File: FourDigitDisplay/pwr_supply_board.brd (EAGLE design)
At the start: 65 x 47 mm, 28 parts, among them CN1 POWER_IF, CN2 POWER_IF, CN3 POWER_IF, Q1 2SA1020L-Y, Q2 2SK3234, U1 MC34063AP1, U5 XC6202P502TB

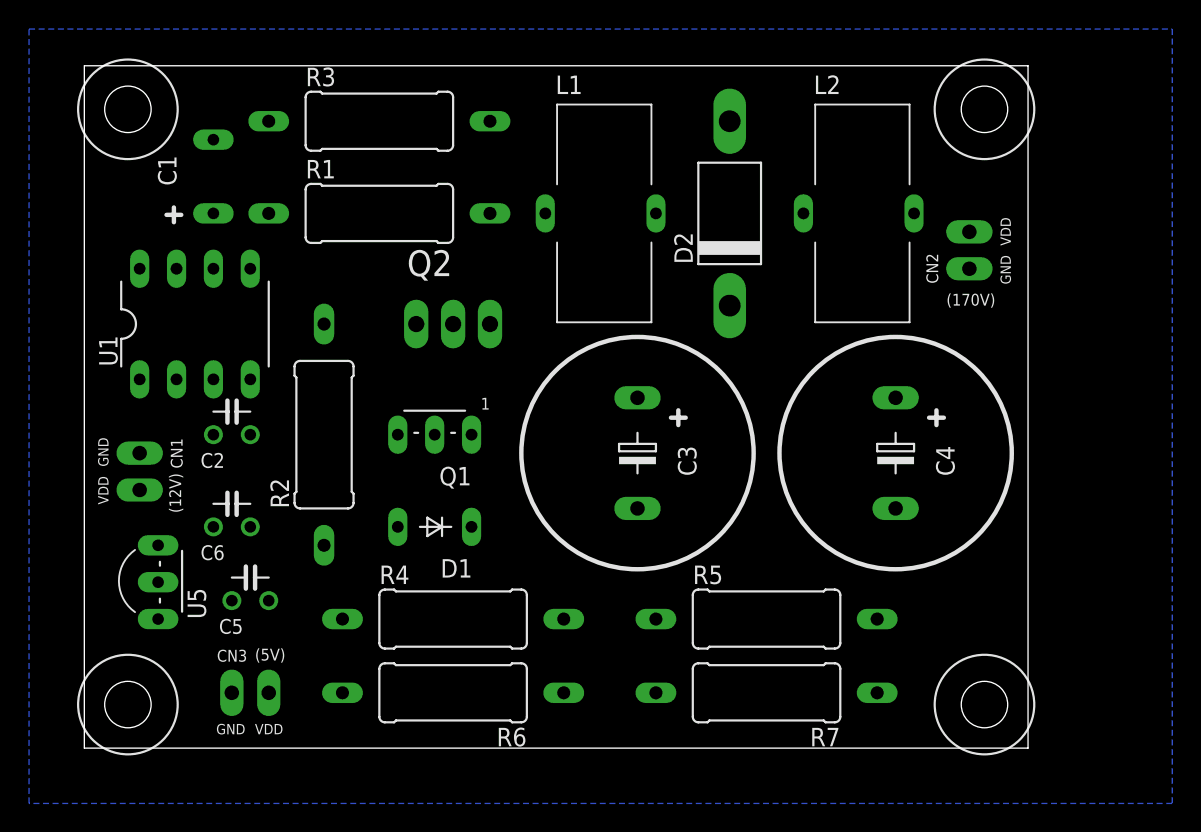
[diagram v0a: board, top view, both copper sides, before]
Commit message: 電源基板の部品配線
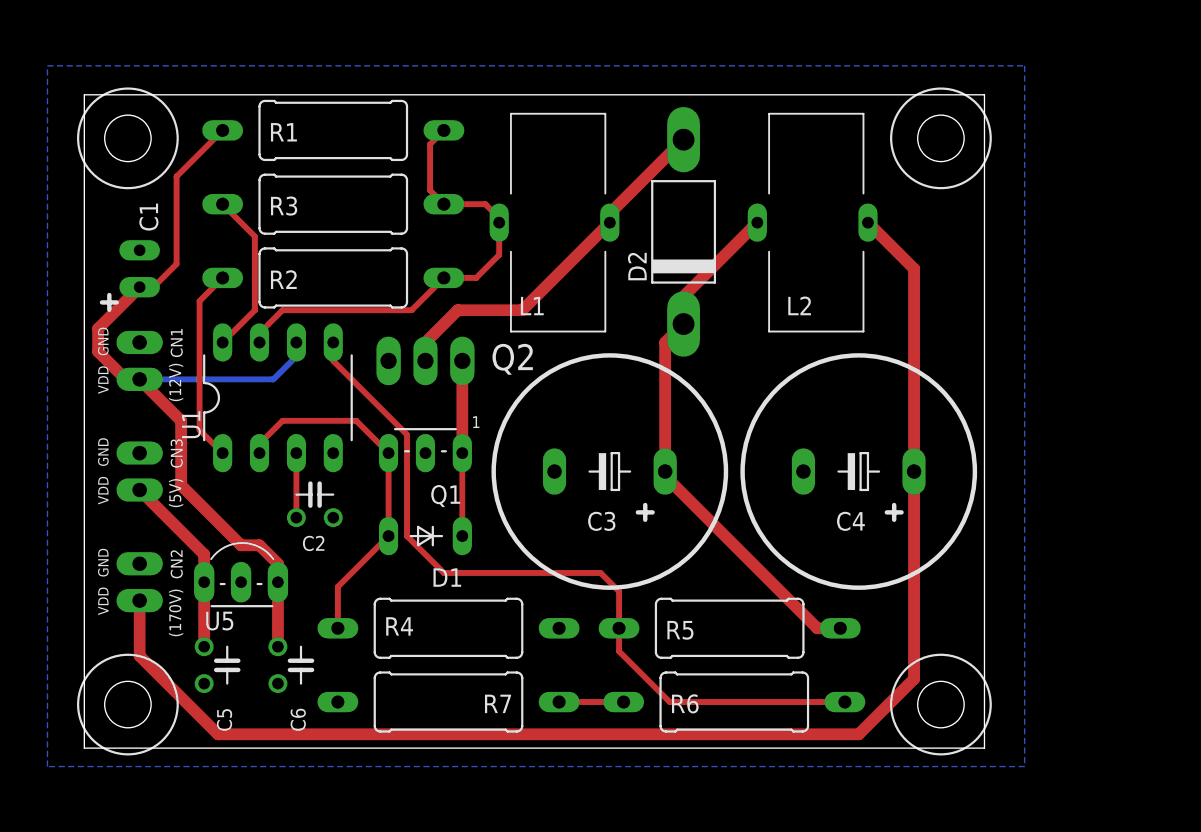
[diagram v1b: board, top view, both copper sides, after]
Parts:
- C1: device Parts:ELECAP_200MIL -> Parts:ELECAP_100MIL
- moved CN2 60.7 mm to (3.81, 12.7), turned to 270 degrees
- moved R7 21.9 mm to (25.1, 3.17), turned to 0 degrees
- moved R6 19.4 mm to (44.8, 3.17), turned to 0 degrees
- moved CN3 17.7 mm to (3.81, 20.3), turned to 270 degrees
- moved R2 10.8 mm to (17.1, 32.4), turned to 0 degrees
- moved C6 10.0 mm to (13.3, 5.71), turned to 270 degrees
- moved C2 8.08 mm to (15.9, 15.9)
- moved U1 7.65 mm to (13.3, 24.1)
- moved CN1 7.62 mm to (3.81, 27.9)
- moved C1 7.18 mm to (3.81, 33.0)
- moved R1 6.54 mm to (17.1, 42.5)
- moved R3 6.54 mm to (17.1, 37.5)
- moved C5 5.46 mm to (8.26, 5.71), turned to 270 degrees
- moved Q2 4.07 mm to (26.0, 26.7), turned to 180 degrees
- moved U5 4.07 mm to (8.26, 11.4), turned to 0 degrees
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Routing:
- net +24V: track 0.00 -> 93.7 mm
- net +12V: track 0.00 -> 58.5 mm
- net N$6: track 0.00 -> 52.8 mm
- net N$2: track 0.00 -> 36.5 mm
- net N$5: track 0.00 -> 32.0 mm
- net N$10: track 0.00 -> 25.2 mm
- net N$7: track 0.00 -> 24.6 mm
- net N$4: track 0.00 -> 13.4 mm
- net +5V: track 0.00 -> 12.6 mm
- net N$8: track 0.00 -> 12.1 mm
- net N$1: track 0.00 -> 11.4 mm
- net N$9: track 0.00 -> 4.45 mm
- net N$3: track 0.00 -> 4.45 mm
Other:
- board size 65 x 47 mm -> 62 x 45 mm
